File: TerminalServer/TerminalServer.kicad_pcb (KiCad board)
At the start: 4 copper layers, 135 x 72 mm, 128 parts, among them J1 RJ45_LED, J10 Conn_01x10_Pin, J11 SI-60118-F, J12 Conn_01x08_Pin, J2 RJ45_LED, J3 RJ45_LED, J4 RJ45_LED, J5 RJ45_LED, J6 RJ45_LED, J7 USB_C_Receptacle_USB2.0_14P, J8 Barrel_Jack_Switch, J9 Conn_PIC_ICSP_ICD, SW1 SW_Push, SW2 SW_SPDT, U1 PIC32MX795F512L-80x-PT, U10 24LC16, U11 ENC28J60x-ML, U12 ESP32-S3-WROOM-1, U2 XR32330EBERTR-F, U3 XR32330EBERTR-F, U4 XR32330EBERTR-F, U5 XR32330EBERTR-F, U6 XR32330EBERTR-F, U7 XR32330EBERTR-F, U9 TPS82130, Y1 ASEMB-8.000MHZ-LC-T, Y2 ASEMB-25.000MHZ-LC-T

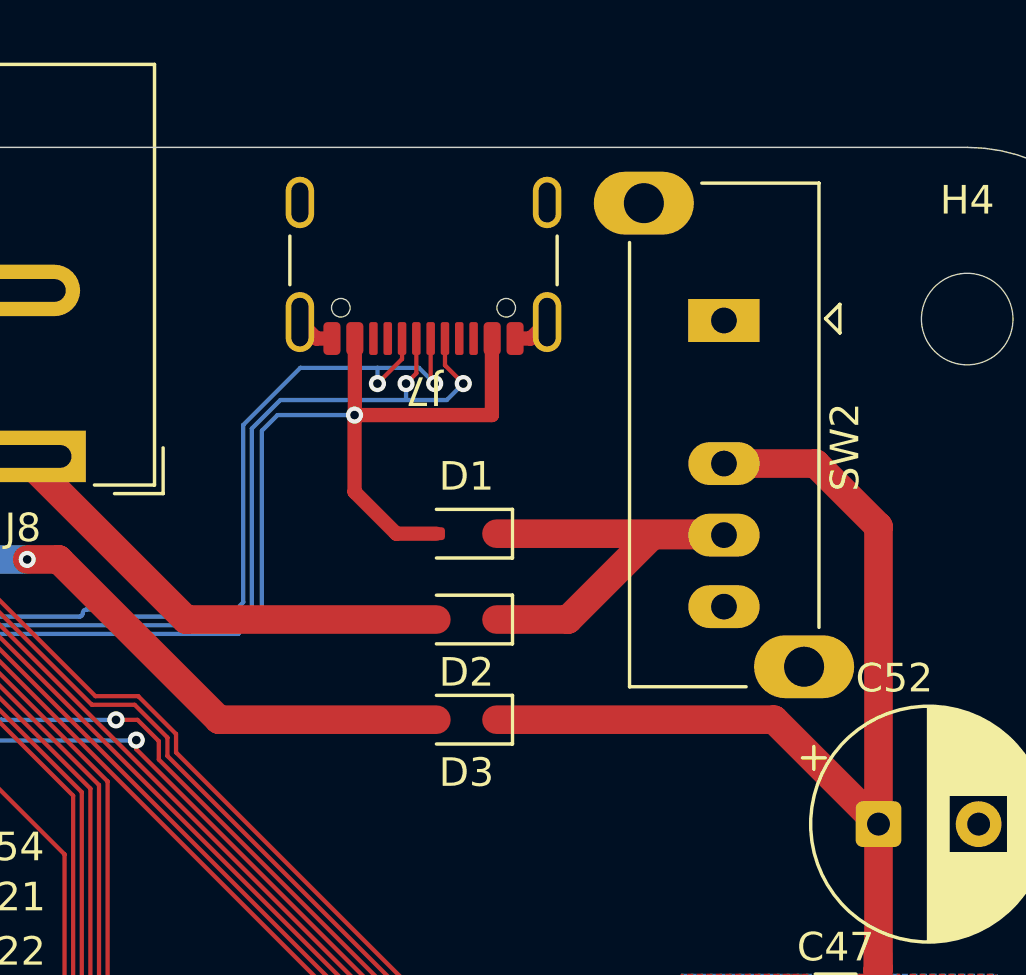
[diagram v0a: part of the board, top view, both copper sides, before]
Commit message: Almost complete
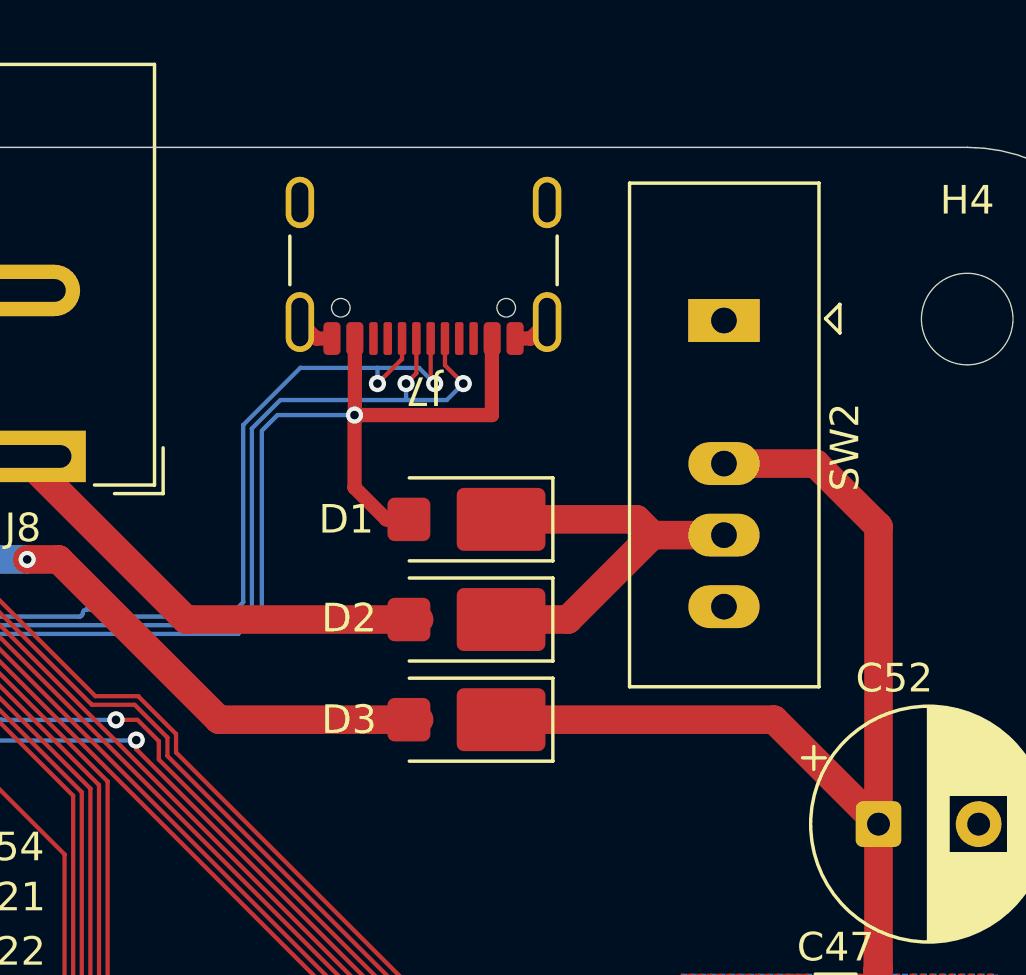
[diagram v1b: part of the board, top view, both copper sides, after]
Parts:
- D1, D2, D3: value 1N5819WS -> V8PAN50-M3/I; footprint Diode_SMD:D_SOD-323 -> Diode_SMD:Vishay_SMPA
- moved D1 0.50 mm to (182.5, 77.0)
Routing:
- net /SWIN: track 17.1 -> 14.2 mm
- net /USB_VBUS: track 59.0 -> 57.7 mm
- net VCC: track 38.3 -> 37.7 mm
- net Net-(D3-A): track 111.8 -> 111.2 mm
- net Net-(D2-A): track 16.8 -> 16.2 mm
